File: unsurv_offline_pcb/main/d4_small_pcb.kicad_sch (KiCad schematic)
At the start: 54 parts, among them J1 U_FL-R-SMT-1_10_, J2 S2B-PH-SM4-TB_LF__SN_, Q1 UMH3N, Q2 Q_PMOS_GSD, U1 TTGO-Micro32-ESP32, U2 MCP73831-2-OT, U3 CAM-M8C-0-10, U4 AP2112K-3.3, U5 CH340G, U6 RF430CL330H, U7 BMA400-I2C, U8 RFM95W-868S2

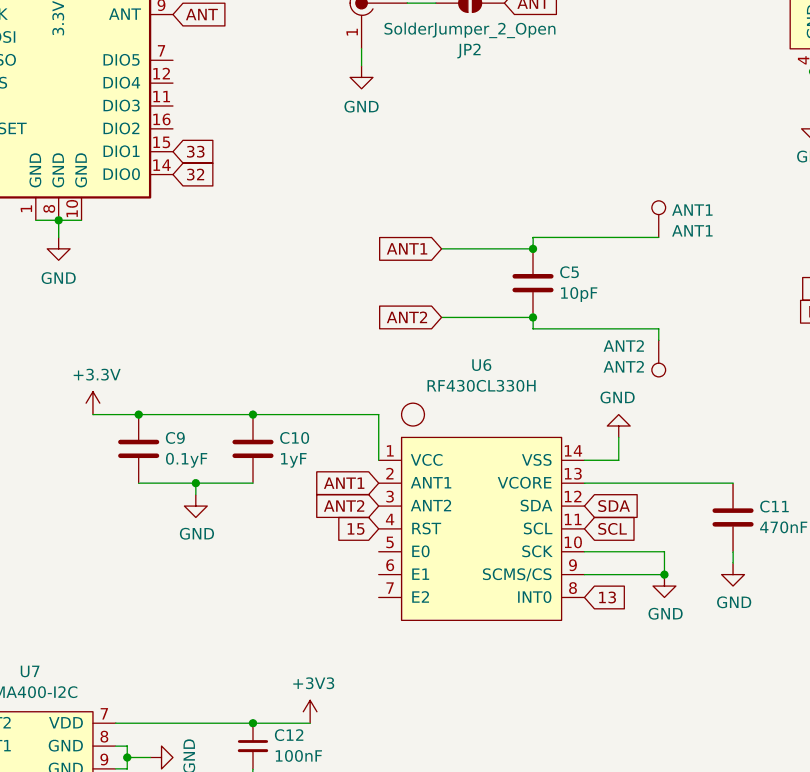
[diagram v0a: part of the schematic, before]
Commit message: v 0.3.1 PCB
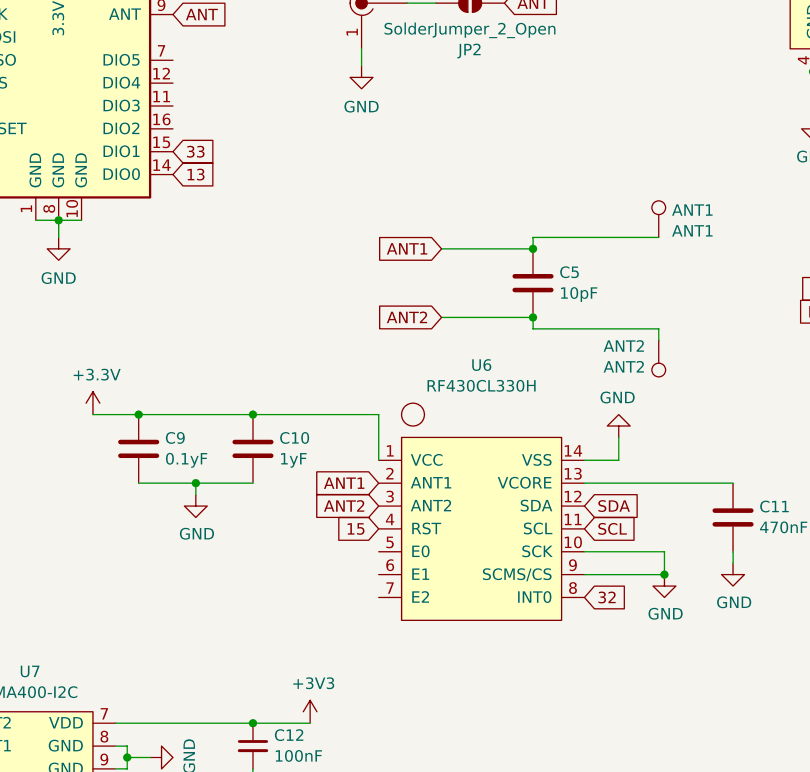
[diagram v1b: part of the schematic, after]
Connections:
- net 13: now also U8.14 (DIO0); no longer U6.8 (INT0)
- net 32: now also U6.8 (INT0); no longer U8.14 (DIO0)
